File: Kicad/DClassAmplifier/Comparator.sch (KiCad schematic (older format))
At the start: 5 parts

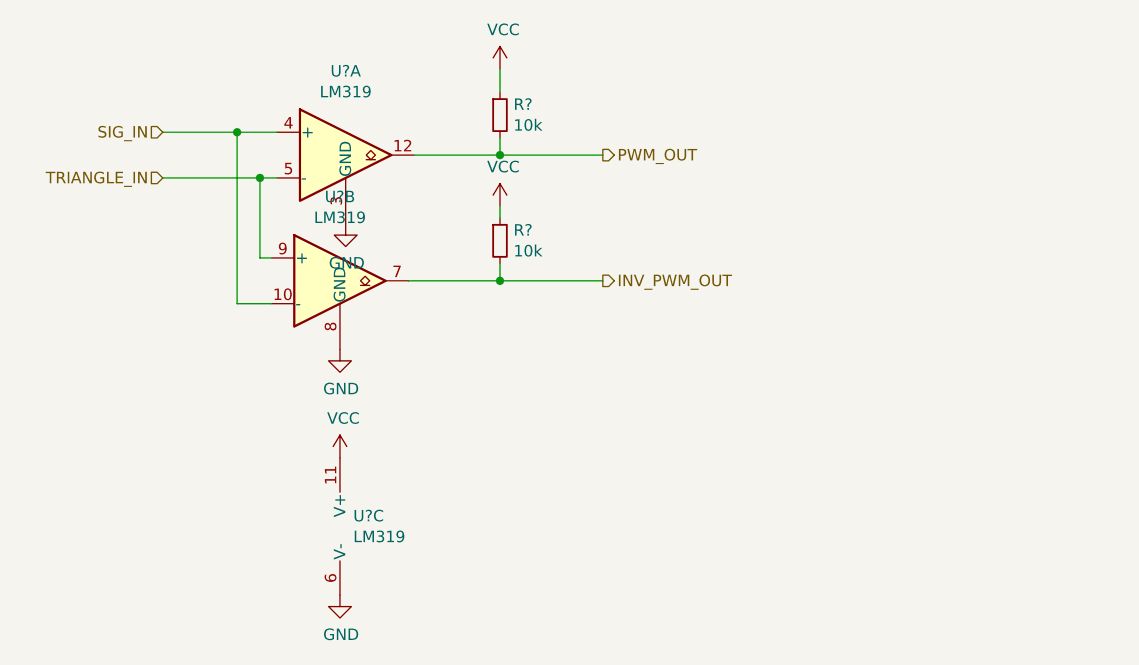
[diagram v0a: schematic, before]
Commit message: updates to schematic
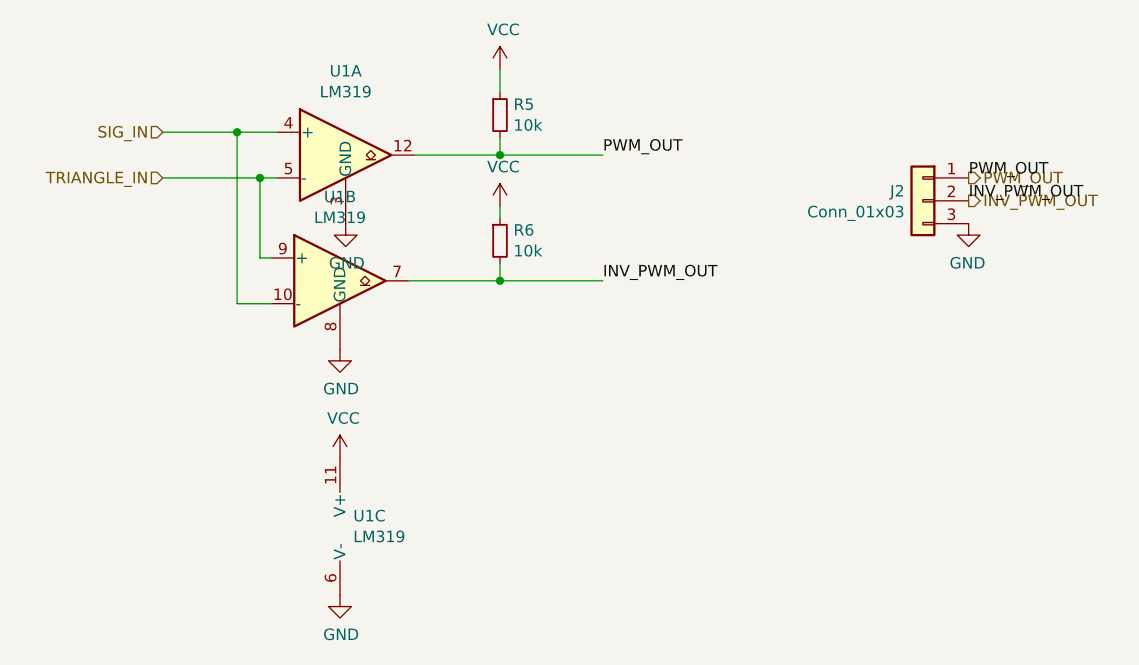
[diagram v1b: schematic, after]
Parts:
- added J2: Conn_01x03, symbol Connector_Generic:Conn_01x03
- R5, R6: renamed from R?; footprint (none) -> Resistor_SMD:R_0603_1608Metric_Pad0.98x0.95mm_HandSolder
- gave numbers to parts that had none: 1
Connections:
- net GND: now also J2.3 (Pin_3)
- net INV_PWM_OUT: now also J2.2 (Pin_2)
- net PWM_OUT: now also J2.1 (Pin_1)
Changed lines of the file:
@@
 $EndDescr
 $Comp
-L Comparator:LM319 U?
+L Comparator:LM319 U1
 U 1 1 61116116
 P 5150 2875
-F 0 "U?" H 5150 3242 50  0000 C CNN
+F 0 "U1" H 5150 3242 50  0000 C CNN
 F 1 "LM319" H 5150 3151 50  0000 C CNN
 F 2 "Package_SO:SO-14_3.9x8.65mm_P1.27mm" H 5150 2875 50  0001 C CNN
@@
 $EndComp
 $Comp
-L Comparator:LM319 U?
+L Comparator:LM319 U1
 U 2 1 6111611C
 P 5125 3425
-F 0 "U?" H 5125 3792 50  0000 C CNN
+F 0 "U1" H 5125 3792 50  0000 C CNN
 F 1 "LM319" H 5125 3701 50  0000 C CNN
 F 2 "Package_SO:SO-14_3.9x8.65mm_P1.27mm" H 5125 3425 50  0001 C CNN
@@
 $EndComp
 $Comp
-L Comparator:LM319 U?
+L Comparator:LM319 U1
 U 3 1 61116122
 P 5225 4500
-F 0 "U?" H 5183 4546 50  0000 L CNN
+F 0 "U1" H 5183 4546 50  0000 L CNN
 F 1 "LM319" H 5183 4455 50  0000 L CNN
 F 2 "Package_SO:SO-14_3.9x8.65mm_P1.27mm" H 5225 4500 50  0001 C CNN
@@
 	1    0    0    -1
 $EndComp
-Wire Wire Line
-	6275 2875 5825 2875
 Wire Wire Line
 	4850 2975 4775 2975
@@
 	4675 3525 4825 3525
 $Comp
-L power:GND #PWR?
+L power:GND #PWR0106
 U 1 1 61116132
 P 5150 3175
-F 0 "#PWR?" H 5150 2925 50  0001 C CNN
+F 0 "#PWR0106" H 5150 2925 50  0001 C CNN
 F 1 "GND" H 5155 3002 50  0000 C CNN
 F 2 "" H 5150 3175 50  0001 C CNN
@@
 $EndComp
 $Comp
-L power:GND #PWR?
+L power:GND #PWR0107
 U 1 1 61116138
 P 5125 3725
-F 0 "#PWR?" H 5125 3475 50  0001 C CNN
+F 0 "#PWR0107" H 5125 3475 50  0001 C CNN
 F 1 "GND" H 5130 3552 50  0000 C CNN
 F 2 "" H 5125 3725 50  0001 C CNN
@@
 $EndComp
 $Comp
-L power:GND #PWR?
+L power:GND #PWR0108
 U 1 1 6111613E
 P 5125 4800
-F 0 "#PWR?" H 5125 4550 50  0001 C CNN
+F 0 "#PWR0108" H 5125 4550 50  0001 C CNN
 F 1 "GND" H 5130 4627 50  0000 C CNN
 F 2 "" H 5125 4800 50  0001 C CNN
@@
 $EndComp
 $Comp
-L power:VCC #PWR?
+L power:VCC #PWR0109
 U 1 1 61116144
 P 5125 4200
-F 0 "#PWR?" H 5125 4050 50  0001 C CNN
+F 0 "#PWR0109" H 5125 4050 50  0001 C CNN
 F 1 "VCC" H 5140 4373 50  0000 C CNN
 F 2 "" H 5125 4200 50  0001 C CNN
@@
 	1    0    0    -1
 $EndComp
-Text HLabel 6275 2875 2    50   Output ~ 0
-PWM_OUT
-Text HLabel 6275 3425 2    50   Output ~ 0
+Text HLabel 7875 3075 2    50   Output ~ 0
 INV_PWM_OUT
 Text HLabel 4350 2975 0    50   Input ~ 0
@@
 	5425 3425 5825 3425
 $Comp
-L Device:R_Small R?
+L Device:R_Small R5
 U 1 1 61119BD5
 P 5825 2700
-F 0 "R?" H 5884 2746 50  0000 L CNN
+F 0 "R5" H 5884 2746 50  0000 L CNN
 F 1 "10k" H 5884 2655 50  0000 L CNN
-F 2 "" H 5825 2700 50  0001 C CNN
+F 2 "Resistor_SMD:R_0603_1608Metric_Pad0.98x0.95mm_HandSolder" H 5825 2700 50  0001 C CNN
 F 3 "~" H 5825 2700 50  0001 C CNN
 	1    5825 2700
@@
 $EndComp
 $Comp
-L Device:R_Small R?
+L Device:R_Small R6
 U 1 1 6111A188
 P 5825 3250
-F 0 "R?" H 5884 3296 50  0000 L CNN
+F 0 "R6" H 5884 3296 50  0000 L CNN
 F 1 "10k" H 5884 3205 50  0000 L CNN
-F 2 "" H 5825 3250 50  0001 C CNN
+F 2 "Resistor_SMD:R_0603_1608Metric_Pad0.98x0.95mm_HandSolder" H 5825 3250 50  0001 C CNN
 F 3 "~" H 5825 3250 50  0001 C CNN
 	1    5825 3250
@@
 $EndComp
 $Comp
-L power:VCC #PWR?
+L power:VCC #PWR0110
 U 1 1 6111A8CA
 P 5825 2500
-F 0 "#PWR?" H 5825 2350 50  0001 C CNN
+F 0 "#PWR0110" H 5825 2350 50  0001 C CNN
 F 1 "VCC" H 5840 2673 50  0000 C CNN
 F 2 "" H 5825 2500 50  0001 C CNN
@@
 $EndComp
 $Comp
-L power:VCC #PWR?
+L power:VCC #PWR0111
 U 1 1 6111AE94
 P 5825 3100
-F 0 "#PWR?" H 5825 2950 50  0001 C CNN
+F 0 "#PWR0111" H 5825 2950 50  0001 C CNN
 F 1 "VCC" H 5840 3273 50  0000 C CNN
 F 2 "" H 5825 3100 50  0001 C CNN
@@
 Wire Wire Line
 	5825 2875 5825 2800
-Connection ~ 5825 2875
 Wire Wire Line
 	5825 2875 5450 2875
@@
 	4775 2975 4350 2975
 Connection ~ 4775 2975
+$Comp
+L Connector_Generic:Conn_01x03 J2
+U 1 1 611080B2
+P 7675 3075
+F 0 "J2" H 7755 3117 50  0000 L CNN
+F 1 "Conn_01x03" H 7755 3026 50  0000 L CNN
+F 2 "" H 7675 3075 50  0001 C CNN
+F 3 "~" H 7675 3075 50  0001 C CNN
+	1    7675 3075
+	-1   0    0    -1
+$EndComp
+Text HLabel 7875 2975 2    50   Output ~ 0
+PWM_OUT
+Connection ~ 5825 2875
+Wire Wire Line
+	6275 2875 5825 2875
+$Comp
+L power:GND #PWR0112
+U 1 1 6110885B
+P 7875 3175
+F 0 "#PWR0112" H 7875 2925 50  0001 C CNN
+F 1 "GND" H 7880 3002 50  0000 C CNN
+F 2 "" H 7875 3175 50  0001 C CNN
+F 3 "" H 7875 3175 50  0001 C CNN
+	1    7875 3175
+	-1   0    0    -1
+$EndComp
+Text Label 7875 2975 0    50   ~ 0
+PWM_OUT
+Text Label 7875 3075 0    50   ~ 0
+INV_PWM_OUT
+Text Label 6275 2875 0    50   ~ 0
+PWM_OUT
+Text Label 6275 3425 0    50   ~ 0
+INV_PWM_OUT
 $EndSCHEMATC
